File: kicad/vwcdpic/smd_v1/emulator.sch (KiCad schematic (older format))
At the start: 38 parts, among them P1 CONN_9, P2 CONN_3, Q1 BC817, Q2 BC807, U1 PIC12F629, U2 78L05, U3 TL072

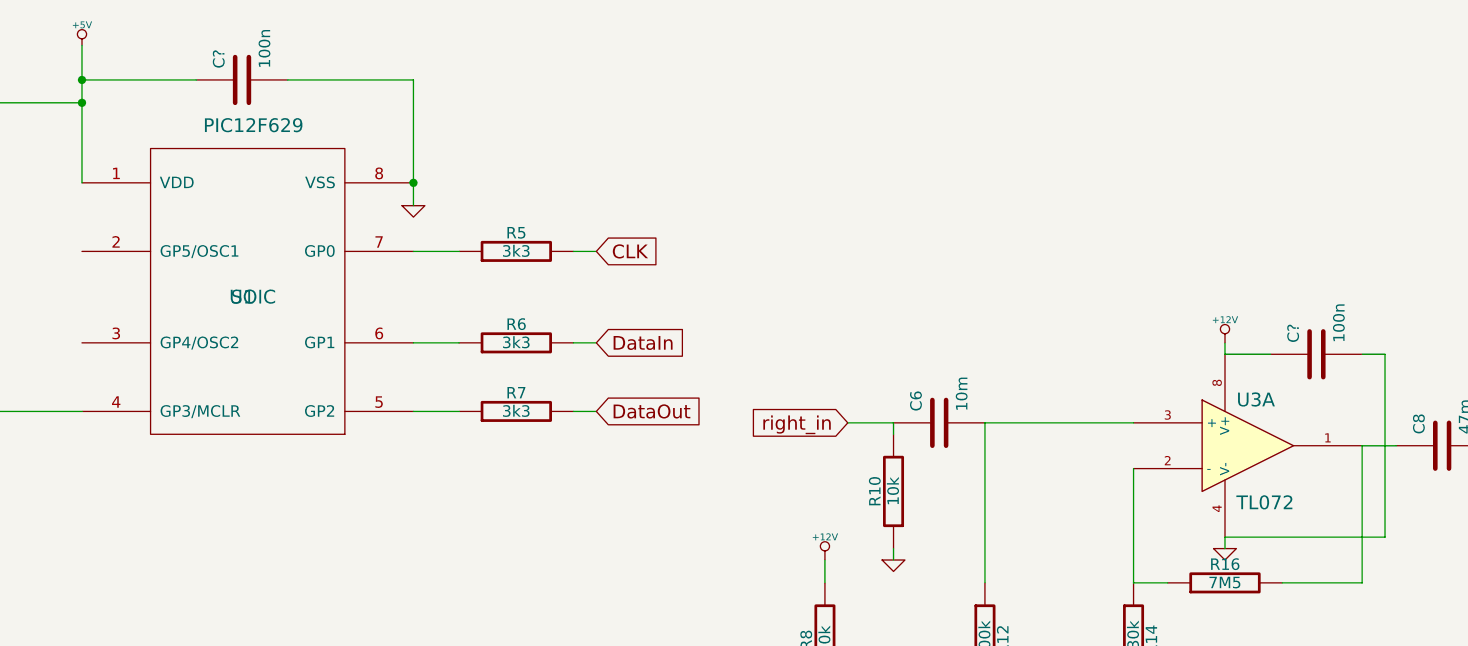
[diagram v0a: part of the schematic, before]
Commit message: garbage cleaning
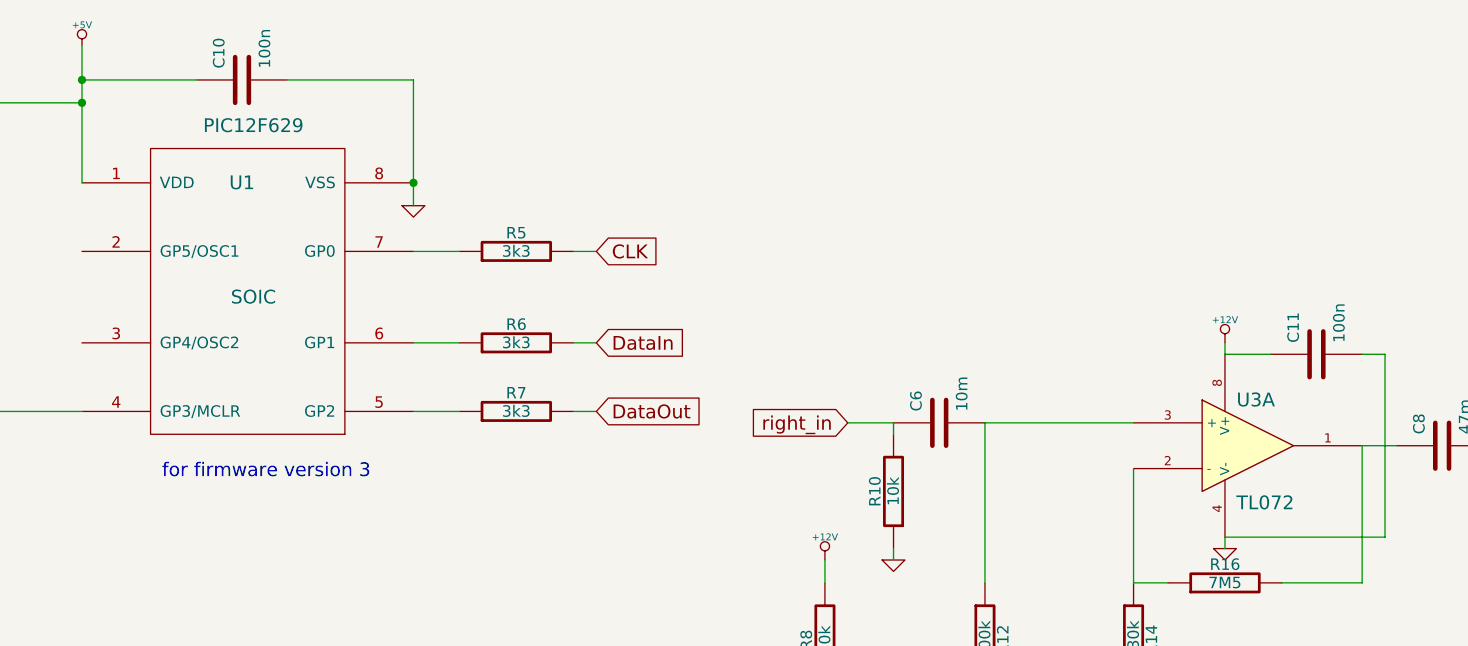
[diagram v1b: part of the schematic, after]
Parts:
- gave numbers to parts that had none: 2
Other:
- note added: "for firmware version 3"
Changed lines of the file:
@@
-EESchema Schematic File Version 2  date Tue 28 Jan 2014 12:56:45 PM CET
+EESchema Schematic File Version 2  date Thu 03 Jul 2014 13:55:33 CEST
 LIBS:power
 LIBS:device
@@
 Sheet 1 1
 Title ""
-Date "28 jan 2014"
+Date "3 jul 2014"
 Rev ""
 Comp ""
@@
 Comment4 ""
 $EndDescr
+Text Notes 2100 2750 0    60   ~ 0
+for firmware version 3
 Wire Wire Line
 	7350 2200 7450 2200
@@
 	6750 2200 6950 2200
 $Comp
-L C C?
+L C C11
 U 1 1 52E79ACE
 P 7150 2200
-F 0 "C?" H 7200 2300 50  0000 L CNN
+F 0 "C11" H 7200 2300 50  0000 L CNN
 F 1 "100n" H 7200 2100 50  0000 L CNN
 	1    7150 2200
@@
 $EndComp
 $Comp
-L C C?
+L C C10
 U 1 1 52E79ABE
 P 2450 1000
-F 0 "C?" H 2500 1100 50  0000 L CNN
+F 0 "C10" H 2500 1100 50  0000 L CNN
 F 1 "100n" H 2500 900 50  0000 L CNN
 	1    2450 1000
@@
 $EndComp
 $Comp
-L GND #PWR01
+L GND #PWR8
 U 1 1 52E774EB
 P 4100 7400
-F 0 "#PWR01" H 4100 7400 30  0001 C CNN
+F 0 "#PWR8" H 4100 7400 30  0001 C CNN
 F 1 "GND" H 4100 7330 30  0001 C CNN
 	1    4100 7400
@@
 $EndComp
 $Comp
-L GND #PWR02
+L GND #PWR11
 U 1 1 52E774E9
 P 5100 7450
-F 0 "#PWR02" H 5100 7450 30  0001 C CNN
+F 0 "#PWR11" H 5100 7450 30  0001 C CNN
 F 1 "GND" H 5100 7380 30  0001 C CNN
 	1    5100 7450
@@
 $EndComp
 $Comp
-L GND #PWR03
+L GND #PWR2
 U 1 1 52E77454
 P 2700 7600
-F 0 "#PWR03" H 2700 7600 30  0001 C CNN
+F 0 "#PWR2" H 2700 7600 30  0001 C CNN
 F 1 "GND" H 2700 7530 30  0001 C CNN
 	1    2700 7600
@@
 $EndComp
 $Comp
-L GND #PWR04
+L GND #PWR4
 U 1 1 52E56B61
 P 3100 7600
-F 0 "#PWR04" H 3100 7600 30  0001 C CNN
+F 0 "#PWR4" H 3100 7600 30  0001 C CNN
 F 1 "GND" H 3100 7530 30  0001 C CNN
 	1    3100 7600
@@
 $EndComp
 $Comp
-L AGND #PWR05
+L AGND #PWR3
 U 1 1 52E56AED
 P 3050 3900
-F 0 "#PWR05" H 3050 3900 40  0001 C CNN
+F 0 "#PWR3" H 3050 3900 40  0001 C CNN
 F 1 "AGND" H 3050 3830 50  0000 C CNN
 	1    3050 3900
@@
 $EndComp
 $Comp
-L GND #PWR06
+L GND #PWR6
 U 1 1 52E56AE2
 P 3750 3900
-F 0 "#PWR06" H 3750 3900 30  0001 C CNN
+F 0 "#PWR6" H 3750 3900 30  0001 C CNN
 F 1 "GND" H 3750 3830 30  0001 C CNN
 	1    3750 3900
@@
 $EndComp
 $Comp
-L AGND #PWR07
+L AGND #PWR23
 U 1 1 52E56AD2
 P 8950 2500
-F 0 "#PWR07" H 8950 2500 40  0001 C CNN
+F 0 "#PWR23" H 8950 2500 40  0001 C CNN
 F 1 "AGND" H 8950 2430 50  0000 C CNN
 	1    8950 2500
@@
 $EndComp
 $Comp
-L AGND #PWR08
+L AGND #PWR22
 U 1 1 52E56ACB
 P 8900 3750
-F 0 "#PWR08" H 8900 3750 40  0001 C CNN
+F 0 "#PWR22" H 8900 3750 40  0001 C CNN
 F 1 "AGND" H 8900 3680 50  0000 C CNN
 	1    8900 3750
@@
 POWER_CTL
 $Comp
-L +12V #PWR09
+L +12V #PWR24
 U 1 1 52D3D406
 P 9100 2650
-F 0 "#PWR09" H 9100 2600 20  0001 C CNN
+F 0 "#PWR24" H 9100 2600 20  0001 C CNN
 F 1 "+12V" H 9100 2750 30  0000 C CNN
 	1    9100 2650
@@
 $EndComp
 $Comp
-L GND #PWR010
+L GND #PWR25
 U 1 1 52D3D3F9
 P 9100 2900
-F 0 "#PWR010" H 9100 2900 30  0001 C CNN
+F 0 "#PWR25" H 9100 2900 30  0001 C CNN
 F 1 "GND" H 9100 2830 30  0001 C CNN
 	1    9100 2900
@@
 right_out
 $Comp
-L GND #PWR011
+L GND #PWR12
 U 1 1 52D3D37E
 P 5300 3100
-F 0 "#PWR011" H 5300 3100 30  0001 C CNN
+F 0 "#PWR12" H 5300 3100 30  0001 C CNN
 F 1 "GND" H 5300 3030 30  0001 C CNN
 	1    5300 3100
@@
 $EndComp
 $Comp
-L GND #PWR012
+L GND #PWR13
 U 1 1 52D3D371
 P 5300 4450
-F 0 "#PWR012" H 5300 4450 30  0001 C CNN
+F 0 "#PWR13" H 5300 4450 30  0001 C CNN
 F 1 "GND" H 5300 4380 30  0001 C CNN
 	1    5300 4450
@@
 $EndComp
 $Comp
-L +12V #PWR013
+L +12V #PWR21
 U 1 1 52D3D248
 P 6750 5400
-F 0 "#PWR013" H 6750 5350 20  0001 C CNN
+F 0 "#PWR21" H 6750 5350 20  0001 C CNN
 F 1 "+12V" H 6750 5500 30  0000 C CNN
 	1    6750 5400
@@
 $EndComp
 $Comp
-L GND #PWR014
+L GND #PWR19
 U 1 1 52D3D240
 P 6750 3050
-F 0 "#PWR014" H 6750 3050 30  0001 C CNN
+F 0 "#PWR19" H 6750 3050 30  0001 C CNN
 F 1 "GND" H 6750 2980 30  0001 C CNN
 	1    6750 3050
@@
 $EndComp
 $Comp
-L GND #PWR015
+L GND #PWR20
 U 1 1 52D3D22F
 P 6750 4500
-F 0 "#PWR015" H 6750 4500 30  0001 C CNN
+F 0 "#PWR20" H 6750 4500 30  0001 C CNN
 F 1 "GND" H 6750 4430 30  0001 C CNN
 	1    6750 4500
@@
 $EndComp
 $Comp
-L +12V #PWR016
+L +12V #PWR18
 U 1 1 52D3D226
 P 6750 2150
-F 0 "#PWR016" H 6750 2100 20  0001 C CNN
+F 0 "#PWR18" H 6750 2100 20  0001 C CNN
 F 1 "+12V" H 6750 2250 30  0000 C CNN
 	1    6750 2150
@@
 $EndComp
 $Comp
-L +12V #PWR017
+L +12V #PWR9
 U 1 1 52D3D180
 P 5000 3100
-F 0 "#PWR017" H 5000 3050 20  0001 C CNN
+F 0 "#PWR9" H 5000 3050 20  0001 C CNN
 F 1 "+12V" H 5000 3200 30  0000 C CNN
 	1    5000 3100
@@
 $EndComp
 $Comp
-L GND #PWR018
+L GND #PWR10
 U 1 1 52D3D179
 P 5000 4450
-F 0 "#PWR018" H 5000 4450 30  0001 C CNN
+F 0 "#PWR10" H 5000 4450 30  0001 C CNN
 F 1 "GND" H 5000 4380 30  0001 C CNN
 	1    5000 4450
@@
 DataIn
 $Comp
-L +12V #PWR019
+L +12V #PWR7
 U 1 1 52D03307
 P 4100 5400
-F 0 "#PWR019" H 4100 5350 20  0001 C CNN
+F 0 "#PWR7" H 4100 5350 20  0001 C CNN
 F 1 "+12V" H 4100 5500 30  0000 C CNN
 	1    4100 5400
@@
 $EndComp
 $Comp
-L +5V #PWR020
+L +5V #PWR1
 U 1 1 52D03030
 P 1750 850
-F 0 "#PWR020" H 1750 940 20  0001 C CNN
+F 0 "#PWR1" H 1750 940 20  0001 C CNN
 F 1 "+5V" H 1750 940 30  0000 C CNN
 	1    1750 850
@@
 $EndComp
 $Comp
-L +5V #PWR021
+L +5V #PWR16
 U 1 1 52D02FCA
 P 6600 6500
-F 0 "#PWR021" H 6600 6590 20  0001 C CNN
+F 0 "#PWR16" H 6600 6590 20  0001 C CNN
 F 1 "+5V" H 6600 6590 30  0000 C CNN
 	1    6600 6500
@@
 $EndComp
 $Comp
-L GND #PWR022
+L GND #PWR5
 U 1 1 52D02FB7
 P 3200 1550
-F 0 "#PWR022" H 3200 1550 30  0001 C CNN
+F 0 "#PWR5" H 3200 1550 30  0001 C CNN
 F 1 "GND" H 3200 1480 30  0001 C CNN
 	1    3200 1550
@@
 $EndComp
 $Comp
-L GND #PWR023
+L GND #PWR15
 U 1 1 52D02FA3
 P 6150 7450
-F 0 "#PWR023" H 6150 7450 30  0001 C CNN
+F 0 "#PWR15" H 6150 7450 30  0001 C CNN
 F 1 "GND" H 6150 7380 30  0001 C CNN
 	1    6150 7450
@@
 $EndComp
 $Comp
-L GND #PWR024
+L GND #PWR14
 U 1 1 52D02FA1
 P 5700 7450
-F 0 "#PWR024" H 5700 7450 30  0001 C CNN
+F 0 "#PWR14" H 5700 7450 30  0001 C CNN
 F 1 "GND" H 5700 7380 30  0001 C CNN
 	1    5700 7450
@@
 $EndComp
 $Comp
-L GND #PWR025
+L GND #PWR17
 U 1 1 52D02F9D
 P 6600 7450
-F 0 "#PWR025" H 6600 7450 30  0001 C CNN
+F 0 "#PWR17" H 6600 7450 30  0001 C CNN
 F 1 "GND" H 6600 7380 30  0001 C CNN
 	1    6600 7450
@@
 U 1 1 52D02953
 P 2500 1950
-F 0 "U1" H 2450 1950 60  0000 C CNN
+F 0 "U1" H 2450 2450 60  0000 C CNN
 F 1 "PIC12F629" H 2500 2700 60  0000 C CNN
 F 2 "SOIC" H 2500 1950 60  0000 C CNN
